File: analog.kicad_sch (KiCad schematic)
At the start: 26 parts, among them J4 Conn_01x04, J5 Conn_01x03, U7 LM4780

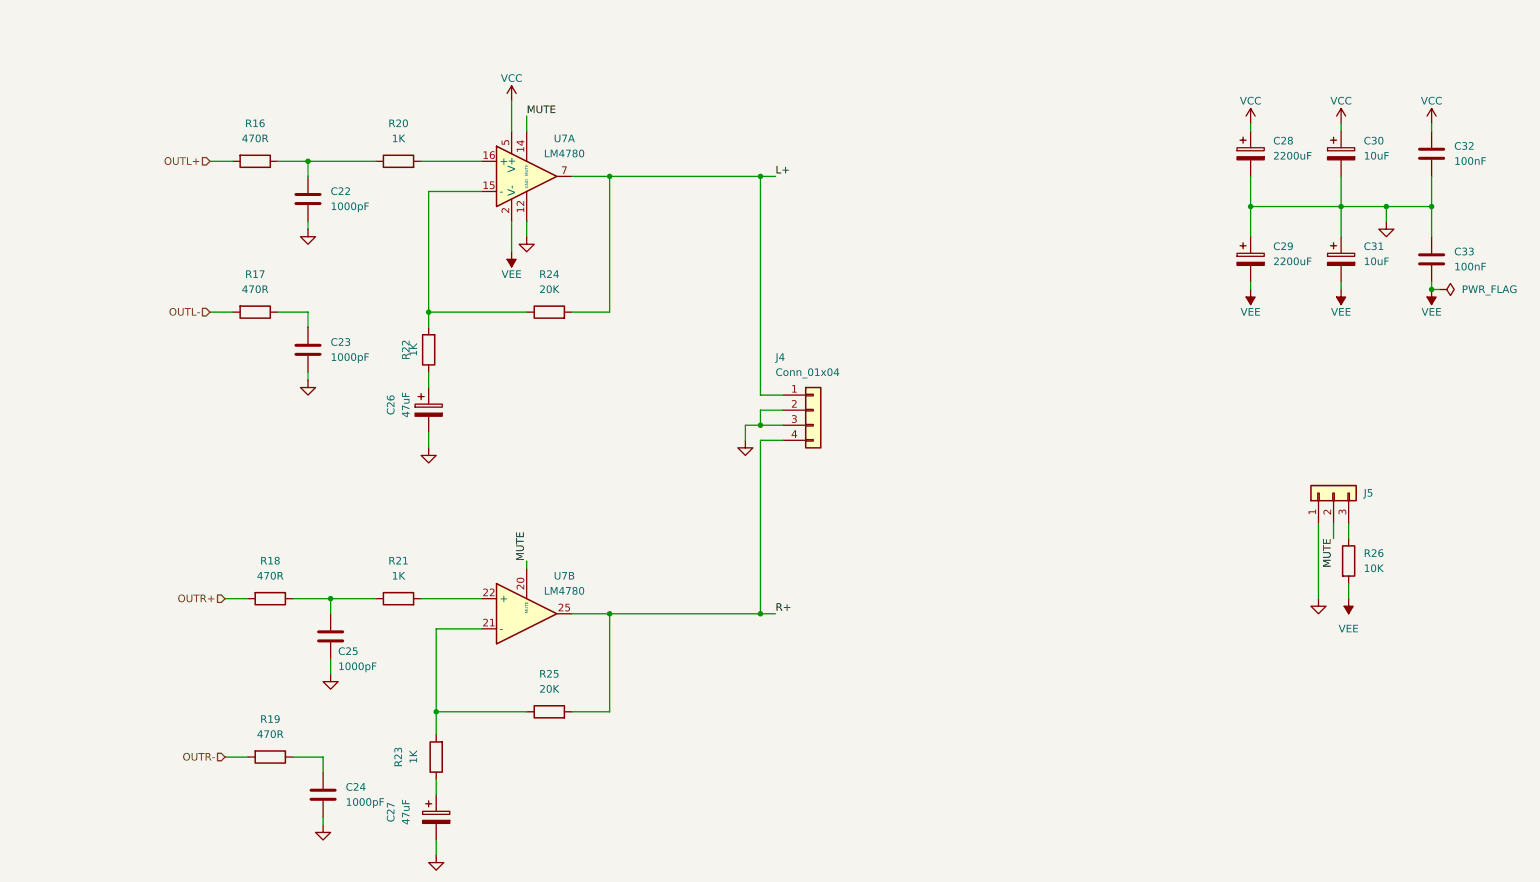
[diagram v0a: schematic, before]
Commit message: WIP
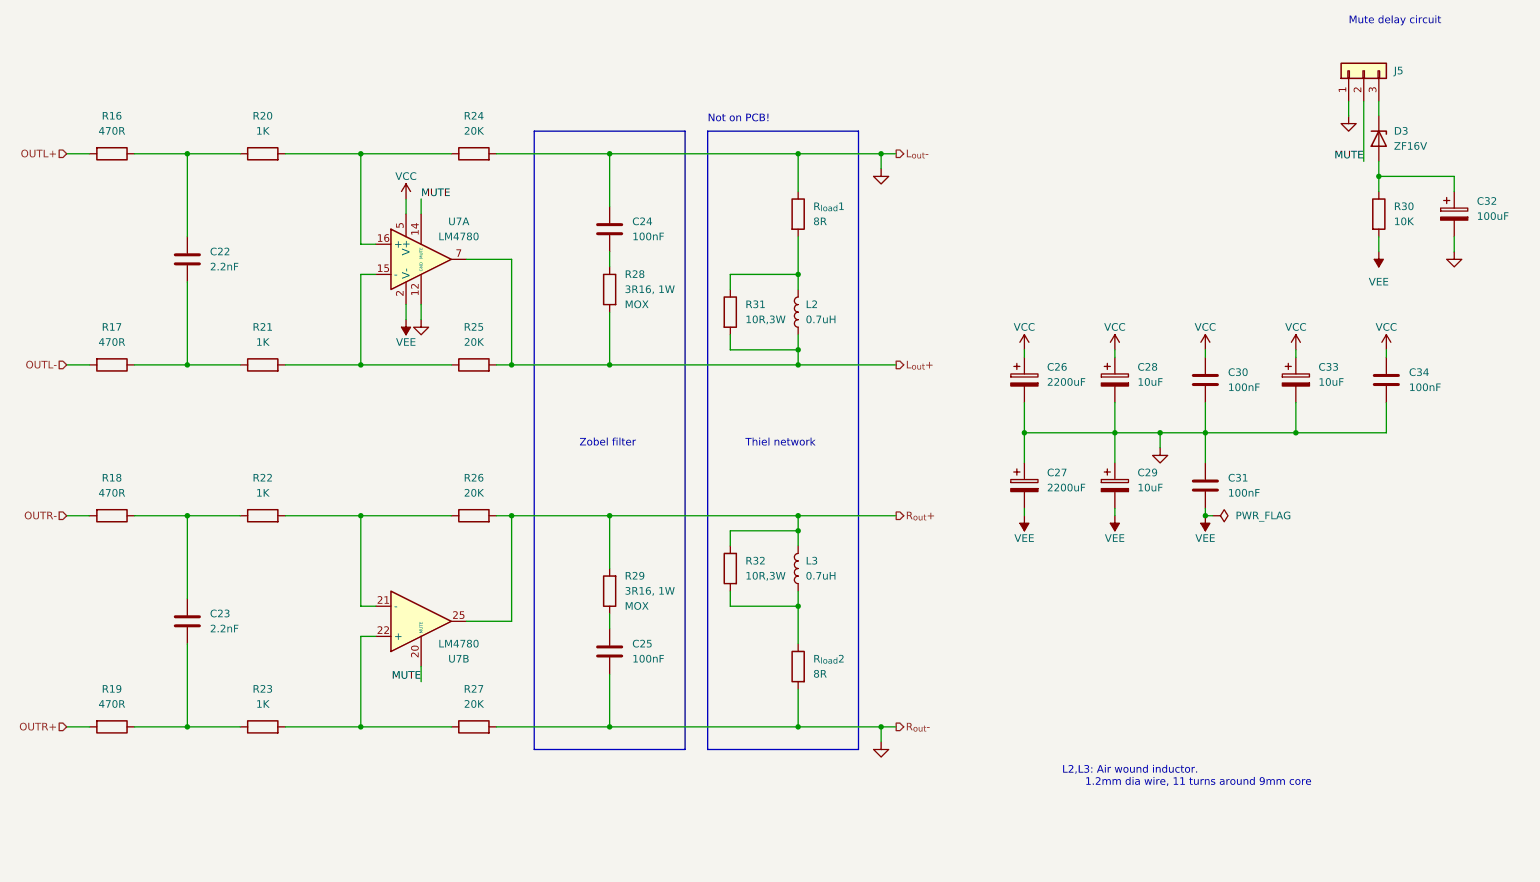
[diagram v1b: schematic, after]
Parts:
- removed C22: 1000pF, Capacitor_SMD:C_0805_2012Metric, symbol Device:C
- removed C26, C27: 47uF, Capacitor_THT:CP_Radial_D6.3mm_P2.50mm, symbol Device:C_Polarized
- removed J4: Conn_01x04, Connector_Phoenix_MSTB:PhoenixContact_MSTBVA_2,5_4-G_1x04_P5.00mm_Vertical, symbol Connector_Generic:Conn_01x04
- added C23: 2.2nF, Capacitor_SMD:C_0805_2012Metric, symbol Device:C
- added C32: 100uF, Capacitor_THT:CP_Radial_D6.3mm_P2.50mm, symbol Device:C_Polarized
- added C33: 10uF, Capacitor_THT:CP_Radial_D6.3mm_P2.50mm, symbol Device:C_Polarized
- added C34: 100nF, Capacitor_THT:C_Rect_L7.2mm_W2.5mm_P5.00mm_FKS2_FKP2_MKS2_MKP2, symbol Device:C
- added D3: ZF16V, Diode_SMD:D_0805_2012Metric, symbol Device:D_Zener
- added L2, L3: 0.7uH, Etnolit:L_Axial_L13.25_D11.4_P13.25_Horizontal, symbol Device:L
- added R26, R27: 20K, Resistor_SMD:R_0805_2012Metric, symbol Device:R
- added R28, R29: 3R16, 1W, Resistor_THT:R_Axial_DIN0309_L9.0mm_D3.2mm_P12.70mm_Horizontal, symbol Device:R
- added R31, R32: 10R,3W, Resistor_THT:R_Axial_DIN0617_L17.0mm_D6.0mm_P20.32mm_Horizontal, symbol Device:R
- added R_{load}1, R_{load}2: 8R, symbol Device:R
- C22: renamed from C23; value 1000pF -> 2.2nF
- C24, C25: value 1000pF -> 100nF; footprint Capacitor_SMD:C_0805_2012Metric -> Capacitor_THT:C_Rect_L7.2mm_W2.5mm_P5.00mm_FKS2_FKP2_MKS2_MKP2
- C30: renamed from C32; footprint Capacitor_SMD:C_0805_2012Metric -> Capacitor_THT:C_Rect_L7.2mm_W2.5mm_P5.00mm_FKS2_FKP2_MKS2_MKP2
- C31: renamed from C33; footprint Capacitor_SMD:C_0805_2012Metric -> Capacitor_THT:C_Rect_L7.2mm_W2.5mm_P5.00mm_FKS2_FKP2_MKS2_MKP2
- R21, R22: footprint Resistor_SMD:R_0805_2012Metric -> Resistor_THT:R_Axial_DIN0207_L6.3mm_D2.5mm_P7.62mm_Horizontal
- renumbered C28 to C26, C29 to C27, C30 to C28, C31 to C29, R26 to R30
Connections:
- net GND: now also R24.2, C32.2, C33.2, C34.2, R27.2, R_{load}1.1, R_{load}2.2; no longer C22.1
- net OUTR+: now also R19.2; no longer R18.2
- net OUTR-: now also R18.2; no longer R19.2
- net VCC: now also C33.1, C34.1
- net at R16.1, R20.1: now also C22.2
- net at R17.1: now also C22.1, R21.1; no longer C22.2
- net at R20.2, U7.16 (+): now also R24.1
- net at R22.1: now also R18.1, C23.2
- net at J5.3 (Pin_3): now also D3.1 (K); no longer R30.1
- net at C24.2: now also R28.1; no longer R19.1
- net at R23.1: now also R19.1, C23.1
- net at R21.2: now also R25.1, U7.15 (-); no longer U7.22 (+)
- net L+ renamed L_{out}+
- net L_{out}+: now also R25.2, L2.1, R28.2, R31.2; no longer R24.2
- net R+ renamed R_{out}+
- net R_{out}+: now also L3.2, R26.2, R29.2, R32.1; no longer R25.2
- new net: L2.2, R31.1, R_{load}1.2
- new net: C25.1, R29.1
- new net: R22.2, R26.1, U7.21 (-)
- new net: L3.1, R32.2, R_{load}2.1
- new net: C32.1, D3.2 (A), R30.1
- new net: R23.2, R27.1, U7.22 (+)
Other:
- note added: "L2,L3: Air wound inductor. 1.2mm dia wire, 11 turns around 9mm core"
- note added: "Mute delay circuit"
- note added: "Not on PCB!"
- note added: "Thiel network"
- note added: "Zobel filter"
- moved on the sheet: C22, C26, C27, C28, C29, C30, C31, J5, R16, R17, R24, R30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
